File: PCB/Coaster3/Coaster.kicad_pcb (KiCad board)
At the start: 2 copper layers, 120 x 120 mm, 279 parts, among them J1 Reset, J2 TC2030-USB-NL-DS, J3 USB-C-Socket-H, J4 DC, J5 DC, U1 ICS43434_MEMS_Mic, U2 ESP32-S3-MINI-1, U3 MD8942

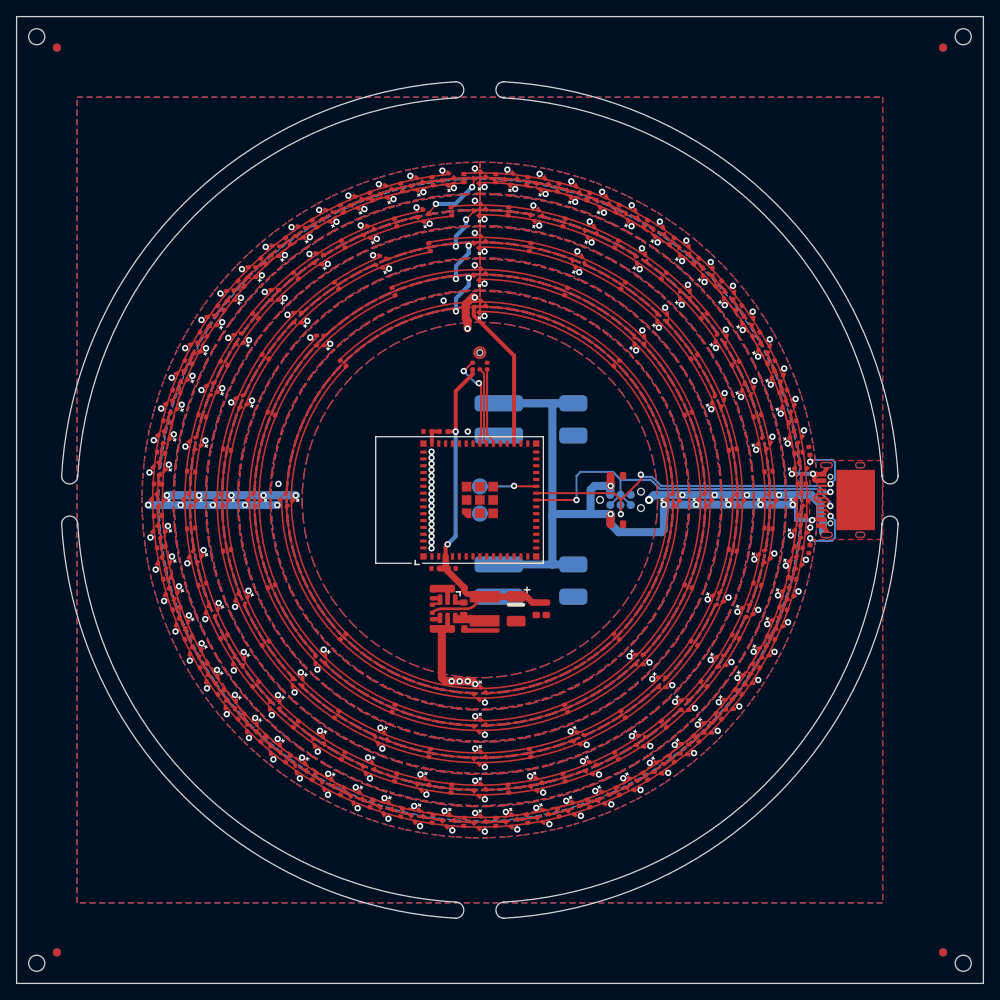
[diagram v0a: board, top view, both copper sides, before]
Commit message: Library update
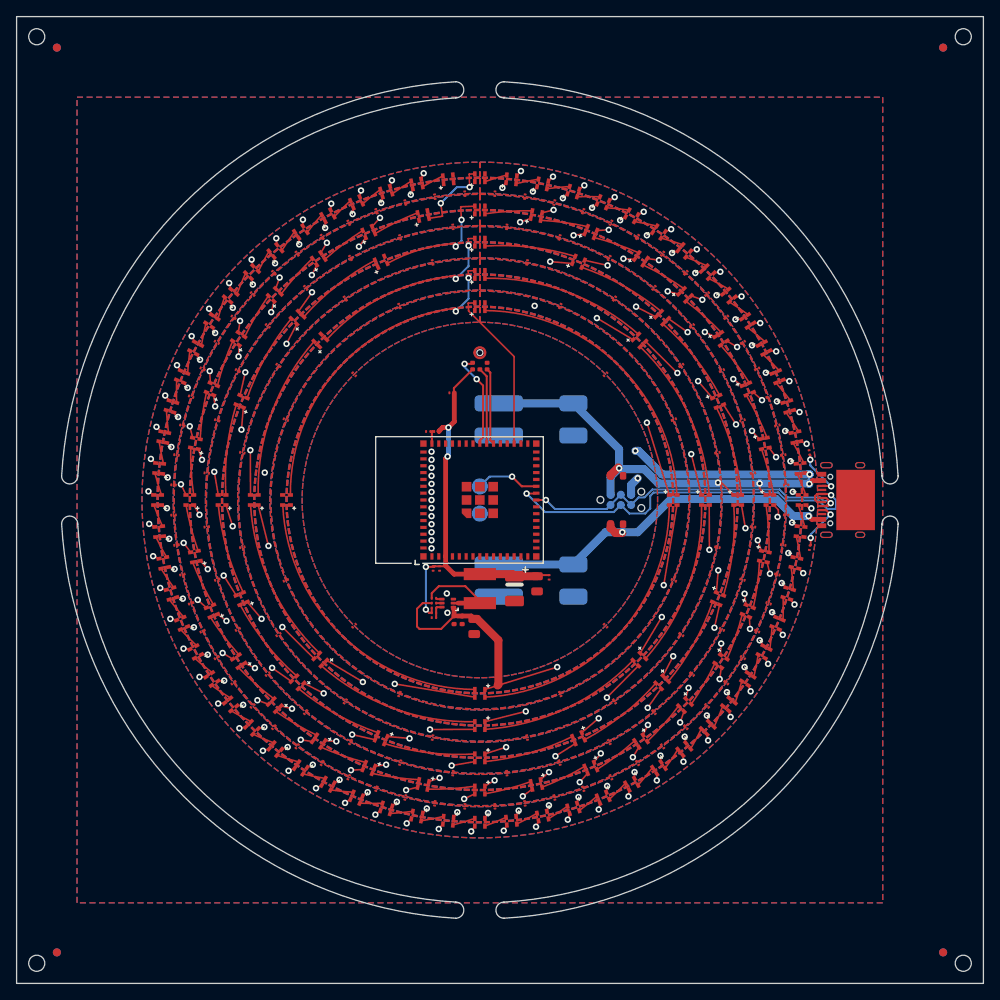
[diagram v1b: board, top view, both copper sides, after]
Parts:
- removed C132: 100nF, RevK:C_0402
- added C127: 220uF Tant, RevK:CP_EIA-3528-21_Kemet-B, F.Cu at (104.3, 111.0)
- added C128: 100nF, RevK:C_0201, F.Cu at (96.5, 86.7)
- added C140: 100nF, RevK:C_0201, F.Cu at (94.2, 108.5)
- added C141: 100nF, RevK:C_0201, F.Cu at (108.6, 109.6)
- C1, C10, C100, C101, C102, C103, C104, C105, C106, C107, C108, C109, C11, C110, C111, C112, C113, C114, C115, C116, C117, C118, C119, C12, C120, C121, C122, C123, C124, C13, C14, C15, C16, C17, C18, C19, C2, C20, C21, C22, C23, C24, C25, C26, C27, C28, C29, C3, C30, C31, C32, C33, C34, C35, C36, C37, C38, C39, C4, C40, C41, C42, C43, C44, C45, C46, C47, C48, C49, C5, C50, C51, C52, C53, C54, C55, C56, C57, C58, C59, C6, C60, C61, C62, C63, C64, C65, C66, C67, C68, C69, C7, C70, C71, C72, C73, C74, C75, C76, C77, C78, C79, C8, C80, C81, C82, C83, C84, C85, C86, C87, C88, C89, C9, C90, C91, C92, C93, C94, C95, C96, C97, C98, C99: footprint RevK:C_0402 -> RevK:C_0201
- C129: value 100nF -> 10uF 35V; footprint RevK:C_0402 -> RevK:C_0603
- C130: value 22uF -> 1uF; footprint RevK:C_0603 -> RevK:C_0201
- C131: value 220uF Tant -> 10uF 35V; footprint RevK:CP_EIA-3528-21_Kemet-B -> RevK:C_0603
- C133: value 10uF 35V -> 22uF 25V; footprint RevK:C_0603 -> RevK:C_0805
- C134: value 1uF -> 100nF 25V
- C135: value 10uF 35V -> 100nF 25V; footprint RevK:C_0603 -> RevK:C_0402
- C136: value 10uF 35V -> 100nF; footprint RevK:C_0603 -> RevK:C_0201
- C137: value 10uF 35V -> 18pF; footprint RevK:C_0603_ -> RevK:C_0201
- C138: value 10uF 6.3V -> 47uF 6V; footprint RevK:C_0603_ -> RevK:C_0805
- C139: footprint RevK:C_0603_ -> RevK:C_0201
- J2: value TC2030-USB-NL-DS -> DC; footprint RevK:Tag-Connect_TC2030-IDC-NL_2x03_P1.27mm_Vertical -> RevK:WAGO-2060-452-998-404
- J3: value USB-C-Socket-H -> DC; footprint RevK:USB-C-Socket-H -> RevK:WAGO-2060-452-998-404; moved to B.Cu
- J4: value DC -> TC2030-USB-NL-DS; footprint RevK:WAGO-2060-452-998-404 -> RevK:Tag-Connect_TC2030-IDC-NL_2x03_P1.27mm_Vertical
- J5: value DC -> USB-C-Socket-H; footprint RevK:WAGO-2060-452-998-404 -> RevK:USB-C-Socket-H; moved to F.Cu
- L1: value 10uH -> 4.7uH; footprint RevK:L_4x4_ -> RevK:L_5x5
- R1: footprint RevK:R_0402 -> RevK:R_0201
- R2: value 124k -> 5K1; footprint RevK:R_0402_ -> RevK:R_0201
- R3: value 39k2 -> 5K1; footprint RevK:R_0402_ -> RevK:R_0201
- R4: value 1M -> 150k 1%; footprint RevK:R_0402_ -> RevK:R_0201
- R5: value 5K1 -> 150k 1%; footprint RevK:R_0402 -> RevK:R_0201
- R6: value 5K1 -> 33k 1%; footprint RevK:R_0402 -> RevK:R_0201
- U3: value MD8942 -> TPS562246; footprint RevK:SOT-23-6-MD8942 -> RevK:SOT-563
- moved R6 51.0 mm to (94.3, 114.6), turned to 180 degrees
- moved R3 50.0 mm to (140.9, 94.1), turned to -81.699 degrees
- moved R2 47.4 mm to (140.9, 105.9), turned to -98.3 degrees
- moved R5 47.2 mm to (94.3, 113.4), turned to 0 degrees
- moved J3 38.3 mm to (107.0, 90.0), turned to 0 degrees
- moved J5 38.3 mm to (144.0, 100.0), turned to 90 degrees
- moved C130 25.8 mm to (93.6, 91.5), turned to 180 degrees
- moved C133 25.7 mm to (99.3, 115.7), turned to -90 degrees
- moved C134 23.6 mm to (96.8, 114.9), turned to -90 degrees
- moved C135 22.6 mm to (97.8, 114.9), turned to -90 degrees
- moved C129 21.2 mm to (117.0, 103.0)
- moved C131 20.7 mm to (117.0, 97.0), turned to 0 degrees
- moved J4 14.5 mm to (117.5, 100.0)
- moved J2 14.5 mm to (107.0, 110.0)
- moved C136 14.0 mm to (94.3, 112.2), turned to 180 degrees
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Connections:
- C129 pad 1: +3V3 -> VBUS
- C130 pad 1: +3V3 -> Net-(U2-EN)
- C131 pad 1: +3V3 -> VBUS
- C134 pad 1: Net-(U2-EN) -> VBUS
- C136 pad 1: +3V3 -> BST
- C136 pad 2: GND -> SW
- C29 pad 1: Net-(D30--) -> VBUS
- C30 pad 1: Net-(D30--) -> VBUS
- D30 pad 3: Net-(D30--) -> VBUS
- J2 pad 1: VBUS -> GND
- J2 pad 2: D- -> VBUS
- J4 pad 1: GND -> VBUS
- J4 pad 2: VBUS -> D-
- R5 pad 1: Net-(J3-CC1) -> +3V3
- R5 pad 2: GND -> FB
- R6 pad 1: GND -> FB
- R6 pad 2: Net-(J3-CC2) -> GND
- U3 pad 1: unconnected-(U3-Pad1)_1 -> VBUS
- U3 pad 2: GND -> SW
- U3 pad 3: unconnected-(U3-Pad3)_1 -> GND
- U3 pad 4: unconnected-(U3-EN-Pad4) -> BST
- U3 pad 5: VBUS -> EN
- U3 pad 6: unconnected-(U3-Pad6) -> FB
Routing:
- net GND: track 1093.5 -> 212.4 mm, vias 144 -> 131
- net VBUS: track 1128.5 -> 301.3 mm, vias 131 -> 119
- net Net-(D11-O) (its old number): track 20.7 -> 0.00 mm
- net Net-(D11-O): track 0.00 -> 20.6 mm
- net Net-(D27-O) (its old number): track 11.3 -> 0.00 mm
- net Net-(D26-O) (its old number): track 11.3 -> 0.00 mm
- net Net-(D23-O) (its old number): track 11.3 -> 0.00 mm
- net Net-(D22-O) (its old number): track 11.3 -> 0.00 mm
- net Net-(D19-O) (its old number): track 11.3 -> 0.00 mm
- net Net-(D18-O) (its old number): track 11.3 -> 0.00 mm
- net Net-(D15-O) (its old number): track 11.3 -> 0.00 mm
- net Net-(D14-O) (its old number): track 11.3 -> 0.00 mm
- net Net-(D25-O) (its old number): track 11.3 -> 0.00 mm
- net Net-(D24-O) (its old number): track 11.3 -> 0.00 mm
- net Net-(D21-O) (its old number): track 11.3 -> 0.00 mm
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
